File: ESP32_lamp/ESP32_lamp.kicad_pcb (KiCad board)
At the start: 2 copper layers, 100 x 100 mm, 23 parts, among them J1 Conn_02x05_Odd_Even, Q1 BSS214NW, Q10 BSS214NW, Q2 BSS214NW, Q3 BSS214NW, Q4 BSS214NW, Q5 BSS214NW, Q6 BSS214NW, Q7 BSS214NW, Q8 BSS214NW, Q9 BSS214NW, U1 ESP32-WROOM-32D, U10 TPS62142, U2 LM2595S-3.3, U3 CP2102N-A01-GQFN28, U4 CP2102N-A01-GQFN24, U5 AAAF5051-05, U6 AAAF5051-05, U7 AAAF5051-05, U9 LM2576S-3.3

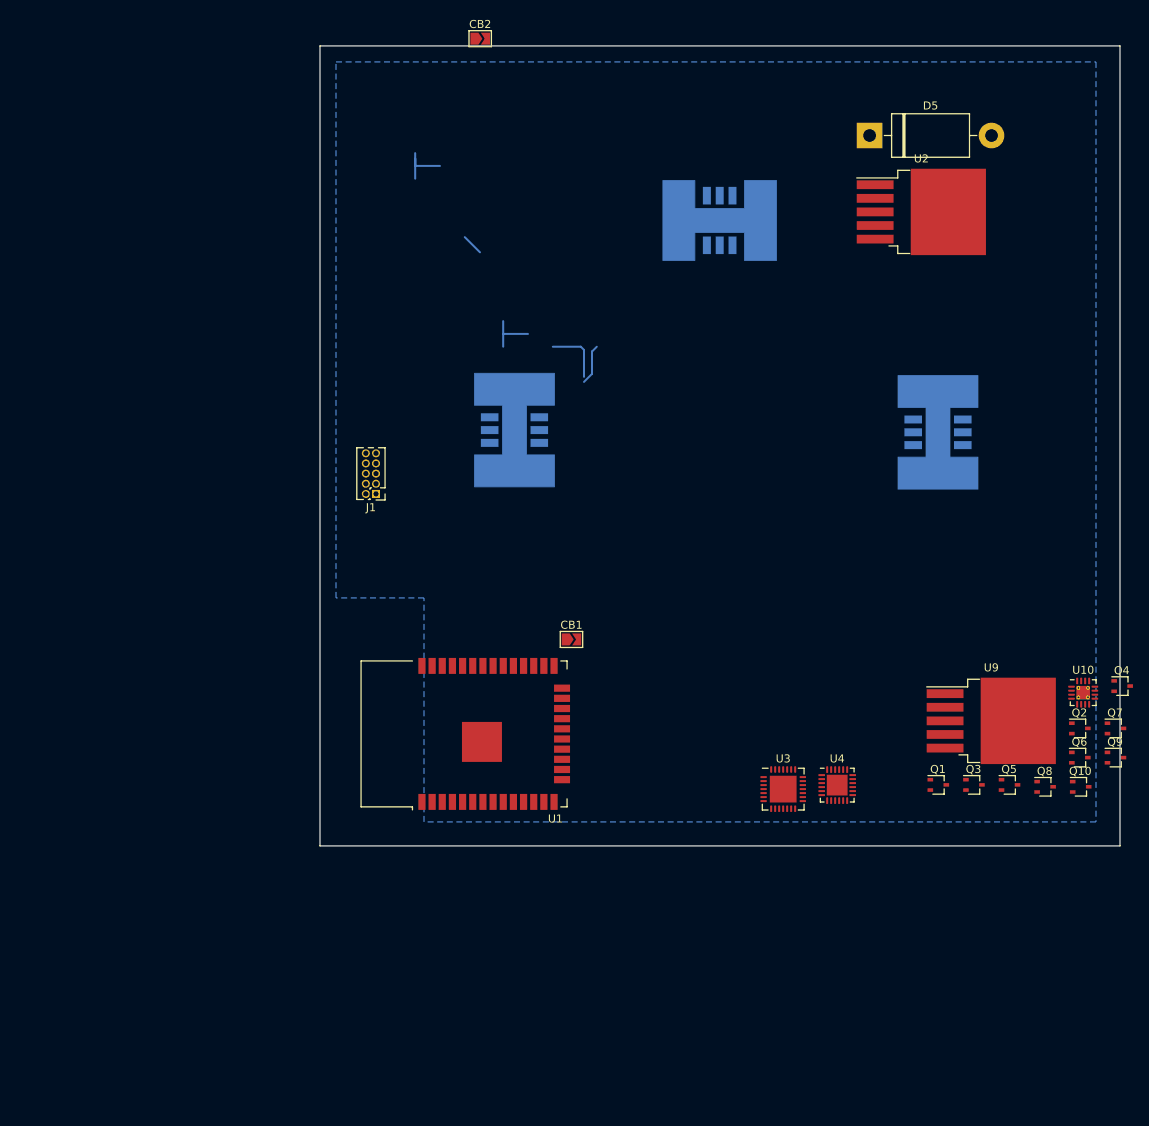
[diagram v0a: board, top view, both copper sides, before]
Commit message: update schem
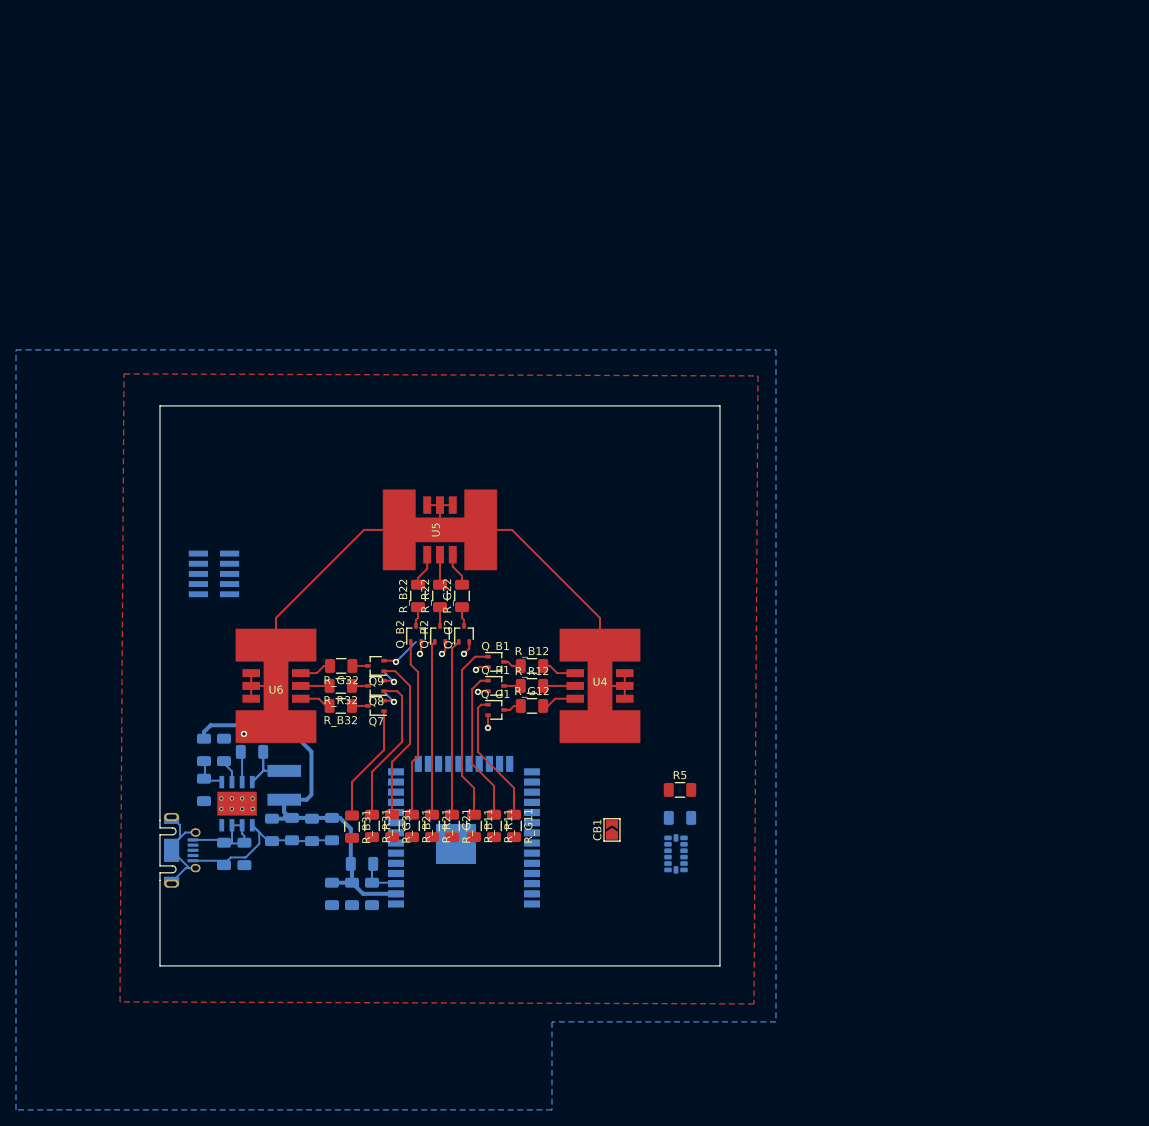
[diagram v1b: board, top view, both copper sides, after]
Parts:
- removed CB2: CircuitBreaker_1P, Jumper:SolderJumper-2_P1.3mm_Open_TrianglePad1.0x1.5mm
- removed D5: 1N5822, Diode_THT:D_DO-201AD_P15.24mm_Horizontal
- removed Q1, Q10, Q2, Q3, Q4, Q5, Q6: BSS214NW, Package_TO_SOT_SMD:SOT-323_SC-70
- removed U10: TPS62142, Package_DFN_QFN:VQFN-16-1EP_3x3mm_P0.5mm_EP1.68x1.68mm_ThermalVias
- removed U7: AAAF5051-05, ESP32_lamp:kinbright-AAAF5051-05
- removed U9: LM2576S-3.3, Package_TO_SOT_SMD:TO-263-5_TabPin3
- added C1: 10uF, Capacitor_SMD:C_1206_3216Metric, B.Cu at (128.0, 131.0)
- added C10: 10uF, Capacitor_SMD:C_1206_3216Metric, B.Cu at (144.0, 136.0)
- added C11: 0.1u, Capacitor_SMD:C_1206_3216Metric, B.Cu at (141.5, 136.0)
- added C2: 220nF, Capacitor_SMD:C_1206_3216Metric, B.Cu at (130.6, 131.0)
- added C3: 1uF, Capacitor_SMD:C_1206_3216Metric, B.Cu at (128.0, 118.0)
- added C4: 100nF, Capacitor_SMD:C_1206_3216Metric, B.Cu at (131.5, 118.2)
- added C5: 22uF, Capacitor_SMD:C_1206_3216Metric, B.Cu at (136.5, 127.9)
- added C6: 22uF, Capacitor_SMD:C_1206_3216Metric, B.Cu at (139.0, 128.0)
- added C7: 22uF, Capacitor_SMD:C_1206_3216Metric, B.Cu at (134.0, 128.0)
- added C8: 22uF, Capacitor_SMD:C_1206_3216Metric, B.Cu at (141.5, 127.9)
- added C9: 0.1uF, Capacitor_SMD:C_1206_3216Metric, B.Cu at (146.5, 136.0)
- added J2: Conn_02x05_Odd_Even, Connector_PinHeader_1.27mm:PinHeader_2x05_P1.27mm_Vertical_SMD, B.Cu at (126.8, 96.0)
- added L1: 2.2uH, 11.4mΩ, Inductor_SMD:L_Taiyo-Yuden_MD-5050, B.Cu at (135.5, 122.4)
- added Q_B1: BSS214NW, Package_TO_SOT_SMD:SOT-323_SC-70, F.Cu at (162.0, 107.0)
- added Q_B2: BSS214NW, Package_TO_SOT_SMD:SOT-323_SC-70, F.Cu at (152.0, 103.5)
- added Q_G1: BSS214NW, Package_TO_SOT_SMD:SOT-323_SC-70, F.Cu at (162.0, 113.0)
- added Q_G2: BSS214NW, Package_TO_SOT_SMD:SOT-323_SC-70, F.Cu at (158.0, 103.5)
- added Q_R1: BSS214NW, Package_TO_SOT_SMD:SOT-323_SC-70, F.Cu at (162.0, 110.0)
- added Q_R2: BSS214NW, Package_TO_SOT_SMD:SOT-323_SC-70, F.Cu at (155.0, 103.5)
- added R1: 100kΩ, Resistor_SMD:R_1206_3216Metric, B.Cu at (125.5, 118.0)
- added R2: 43.3kΩ, Resistor_SMD:R_1206_3216Metric, B.Cu at (125.5, 123.0)
- added R3: 10k, Resistor_SMD:R_1206_3216Metric, B.Cu at (145.2, 132.2)
- added R4: 10k, Resistor_SMD:R_1206_3216Metric, B.Cu at (185.0, 126.5)
- added R5: 10k, Resistor_SMD:R_1206_3216Metric, F.Cu at (185.0, 123.0)
- added R_B11: 220R, Resistor_SMD:R_1206_3216Metric, F.Cu at (159.2, 127.5)
- added R_B12: 0R, Resistor_SMD:R_1206_3216Metric, F.Cu at (166.5, 107.5)
- added R_B21: 220R, Resistor_SMD:R_1206_3216Metric, F.Cu at (151.5, 127.5)
- added R_B22: 0R, Resistor_SMD:R_1206_3216Metric, F.Cu at (152.2, 98.8)
- added R_B31: 220R, Resistor_SMD:R_1206_3216Metric, F.Cu at (144.0, 127.6)
- added R_B32: 0R, Resistor_SMD:R_1206_3216Metric, F.Cu at (142.6, 112.5)
- added R_G11: 220R, Resistor_SMD:R_1206_3216Metric, F.Cu at (164.2, 127.5)
- added R_G12: 0R, Resistor_SMD:R_1206_3216Metric, F.Cu at (166.5, 112.5)
- added R_G21: 220R, Resistor_SMD:R_1206_3216Metric, F.Cu at (156.5, 127.5)
- added R_G22: 0R, Resistor_SMD:R_1206_3216Metric, F.Cu at (157.8, 98.8)
- added R_G31: 220R, Resistor_SMD:R_1206_3216Metric, F.Cu at (149.0, 127.5)
- added R_G32: 0R, Resistor_SMD:R_1206_3216Metric, F.Cu at (142.7, 107.5)
- added R_R11: 220R, Resistor_SMD:R_1206_3216Metric, F.Cu at (161.8, 127.5)
- added R_R12: 6.8R, Resistor_SMD:R_1206_3216Metric, F.Cu at (166.5, 110.0)
- added R_R21: 220R, Resistor_SMD:R_1206_3216Metric, F.Cu at (154.0, 127.5)
- added R_R22: 6.8R, Resistor_SMD:R_1206_3216Metric, F.Cu at (155.0, 98.8)
- added R_R31: 220R, Resistor_SMD:R_1206_3216Metric, F.Cu at (146.5, 127.5)
- added R_R32: 6.8R, Resistor_SMD:R_1206_3216Metric, F.Cu at (142.6, 110.0)
- J1: value Conn_02x05_Odd_Even -> USB_B_Micro; footprint Connector_PinHeader_1.27mm:PinHeader_2x05_P1.27mm_Vertical -> Connector_USB:USB_Micro-AB_Molex_47590-0001; moved to B.Cu
- U1: value ESP32-WROOM-32D -> LMR33630BDDA; footprint RF_Module:ESP32-WROOM-32 -> Package_SO:Texas_HSOP-8-1EP_3.9x4.9mm_P1.27mm_ThermalVias; moved to B.Cu
- U2: value LM2595S-3.3 -> ESP32-WROOM-32D; footprint Package_TO_SOT_SMD:TO-263-5_TabPin3 -> RF_Module:ESP32-WROOM-32; moved to B.Cu
- U3: value CP2102N-A01-GQFN28 -> ADXL343; footprint Package_DFN_QFN:QFN-28-1EP_5x5mm_P0.5mm_EP3.35x3.35mm -> Package_LGA:LGA-14_3x5mm_P0.8mm_LayoutBorder1x6y; moved to B.Cu
- U4: value CP2102N-A01-GQFN24 -> AAAF5051-05; footprint Package_DFN_QFN:QFN-24-1EP_4x4mm_P0.5mm_EP2.6x2.6mm -> ESP32_lamp:kinbright-AAAF5051-05
- U5, U6: moved to F.Cu
- moved U2 96.9 mm to (158.0, 129.0)
- moved Q9 93.1 mm to (147.0, 107.5), turned to 180 degrees
- moved Q7 92.5 mm to (147.0, 112.5), turned to 180 degrees
- moved Q8 84.6 mm to (147.0, 110.0), turned to 180 degrees
- moved U6 80.4 mm to (134.5, 110.0), turned to 0 degrees
- moved J1 51.4 mm to (121.5, 130.6), turned to 90 degrees
- moved U1 32.6 mm to (129.6, 124.7)
- moved U4 32.1 mm to (175.0, 110.0), turned to 180 degrees
- moved CB1 24.3 mm to (176.5, 128.0), turned to 90 degrees
- moved U3 15.7 mm to (184.5, 131.0), turned to 180 degrees
- moved U5 15.6 mm to (155.0, 90.5), turned to 270 degrees
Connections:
- net Net-(U3-Pad8) renamed INT1
- net Net-(U3-Pad9) renamed INT2
- J1 pad 1: +3V3 -> VIN
- J1 pad 2: MTMS -> Net-(J1-Pad2)
- J1 pad 3: GND -> Net-(J1-Pad3)
- J1 pad 4: MTCK -> Net-(J1-Pad4)
- J1 pad 6: MTDO -> GND
- U1 pad 2: +3V3 -> VIN
- U1 pad 3: Net-(U1-Pad3) -> VIN
- U1 pad 9: Net-(U1-Pad9) -> GND
- U2 pad 1: Net-(D5-Pad1) -> GND
- U2 pad 2: +12V -> 3V3
- U2 pad 3: GND -> Net-(C9-Pad2)
- U2 pad 4: +3V3 -> Net-(U2-Pad4)
- U2 pad 5: GND -> Net-(U2-Pad5)
- U3 pad 1: Net-(U3-Pad1) -> 3V3
- U3 pad 11: Net-(U3-Pad11) -> GND
- U3 pad 12: Net-(U3-Pad12) -> GND
- U3 pad 13: Net-(U3-Pad13) -> SDA
- U3 pad 14: Net-(U3-Pad14) -> SCL
- U3 pad 2: Net-(U3-Pad2) -> GND
- U3 pad 3: Net-(U3-Pad29) -> 3V3
- U3 pad 4: Net-(U3-Pad4) -> GND
- U3 pad 5: Net-(U3-Pad5) -> GND
- U3 pad 6: Net-(U3-Pad6) -> 3V3
- U3 pad 7: Net-(U3-Pad7) -> 3V3
- U4 pad 4: Net-(U4-Pad4) -> 3V3_SW
- U4 pad 5: Net-(U4-Pad5) -> 3V3_SW
- U4 pad 6: Net-(U4-Pad6) -> 3V3_SW
- U4 pad 7: Net-(U4-Pad7) -> 3V3_SW
- U5 pad 4: +3V3 -> 3V3_SW
- U5 pad 5: +3V3 -> 3V3_SW
- U5 pad 6: +3V3 -> 3V3_SW
- U5 pad 7: +3V3 -> 3V3_SW
- U6 pad 3: Net-(Q7-Pad3) -> Net-(R_G32-Pad2)
- U6 pad 4: +3V3 -> 3V3_SW
- U6 pad 5: +3V3 -> 3V3_SW
- U6 pad 6: +3V3 -> 3V3_SW
- U6 pad 7: +3V3 -> 3V3_SW
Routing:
- net 3V3_SW: track 0.00 -> 85.5 mm, vias 0 -> 1
- net 3V3: track 0.00 -> 61.3 mm
- net GND: track 0.00 -> 59.9 mm, vias 0 -> 9
- net +3V3: track 23.3 -> 0.00 mm
- net Net-(Q_B1-Pad1): track 0.00 -> 22.7 mm
- net Net-(Q_B2-Pad1): track 0.00 -> 22.3 mm
- net Net-(Q_G2-Pad1): track 0.00 -> 22.0 mm
- net Net-(Q_R2-Pad1): track 0.00 -> 21.7 mm
- net Net-(Q9-Pad1): track 0.00 -> 21.0 mm
- net Net-(Q_R1-Pad1): track 0.00 -> 19.2 mm
- net Net-(Q8-Pad1): track 0.00 -> 18.9 mm
- net Net-(Q_G1-Pad1): track 0.00 -> 16.6 mm
- net Net-(Q7-Pad1): track 0.00 -> 14.7 mm
- net VIN: track 0.00 -> 12.6 mm
- net Net-(C4-Pad1): track 0.00 -> 11.8 mm
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- added copper zone on F.Cu, net 3V3
- added copper zone on B.Cu, net GND
- removed copper zone on B.Cu, net +3V3
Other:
- board size 100 x 100 mm -> 70 x 70 mm
- net class mediomm added: clearance 0.2, trace_width 0.5, via_dia 0.8, via_drill 0.4
